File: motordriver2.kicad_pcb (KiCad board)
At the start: 2 copper layers, 99.7 x 79.7 mm, 129 parts, among them J1 Conn_01x02_Pin, J2 SUB-DRAM-602A-002, J3 SUB-DRAM-602A-002, J4 Conn_01x06_Pin, J5 Conn_01x03_Pin, M1 Motor_DC, Q1 TPHR9003NL, Q2 TPHR9003NL, Q3 TPHR9003NL, Q4 TPHR9003NL, SW1 TS-1187A-B-A-B, SW2 TS-1187A-B-A-B, SW3 TS-1187A-B-A-B, SW4 TS-1187A-B-A-B, SW5 TS-1187A-B-A-B, U1 SN65HVD234, U2 PLM2105DR, U3 STM32F302C8Tx, U4 24LC256, U5 PLM2105DR, U6 AMS1117-3.3, U7 AMS1117-3.3, Y1 Q13FC1350000400, Y2 X322516MLB4SI

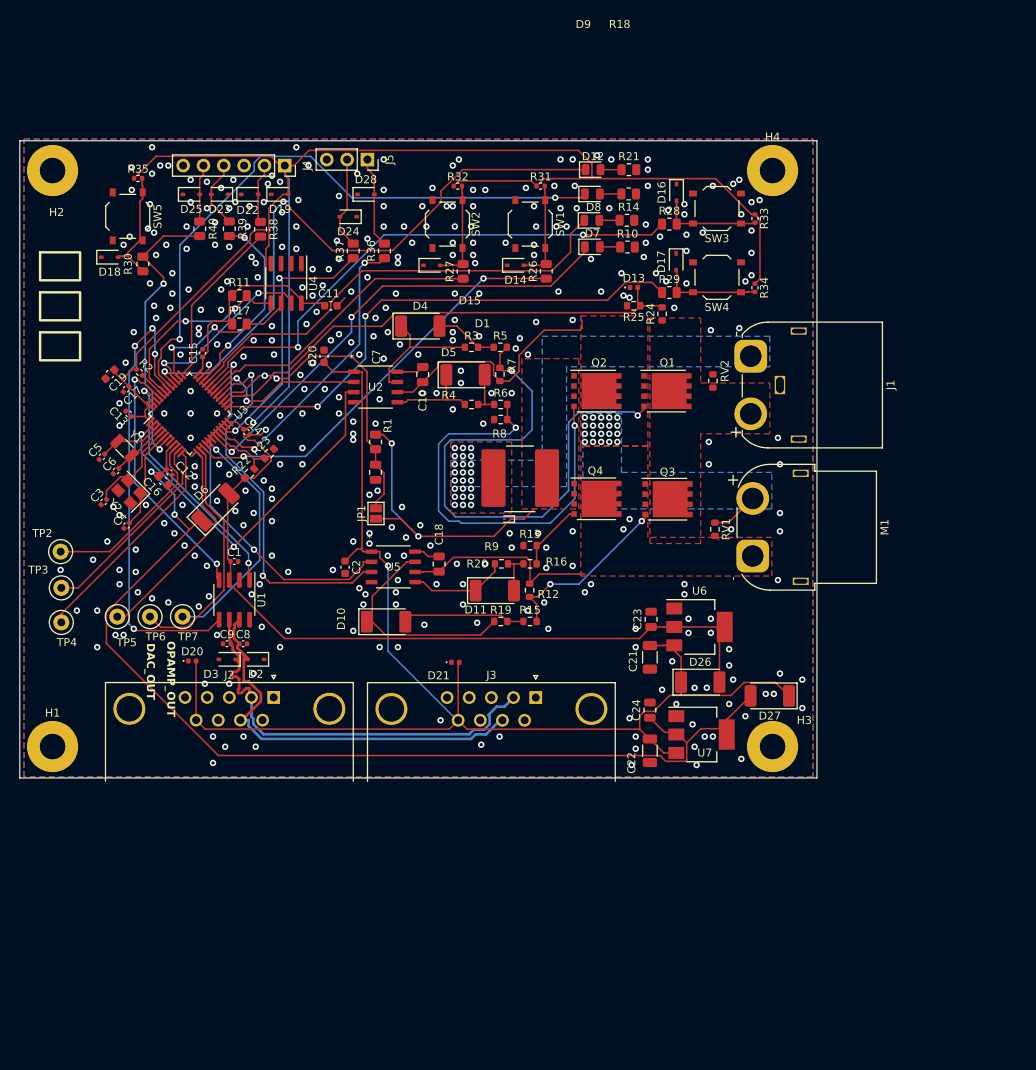
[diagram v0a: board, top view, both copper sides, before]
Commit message: change
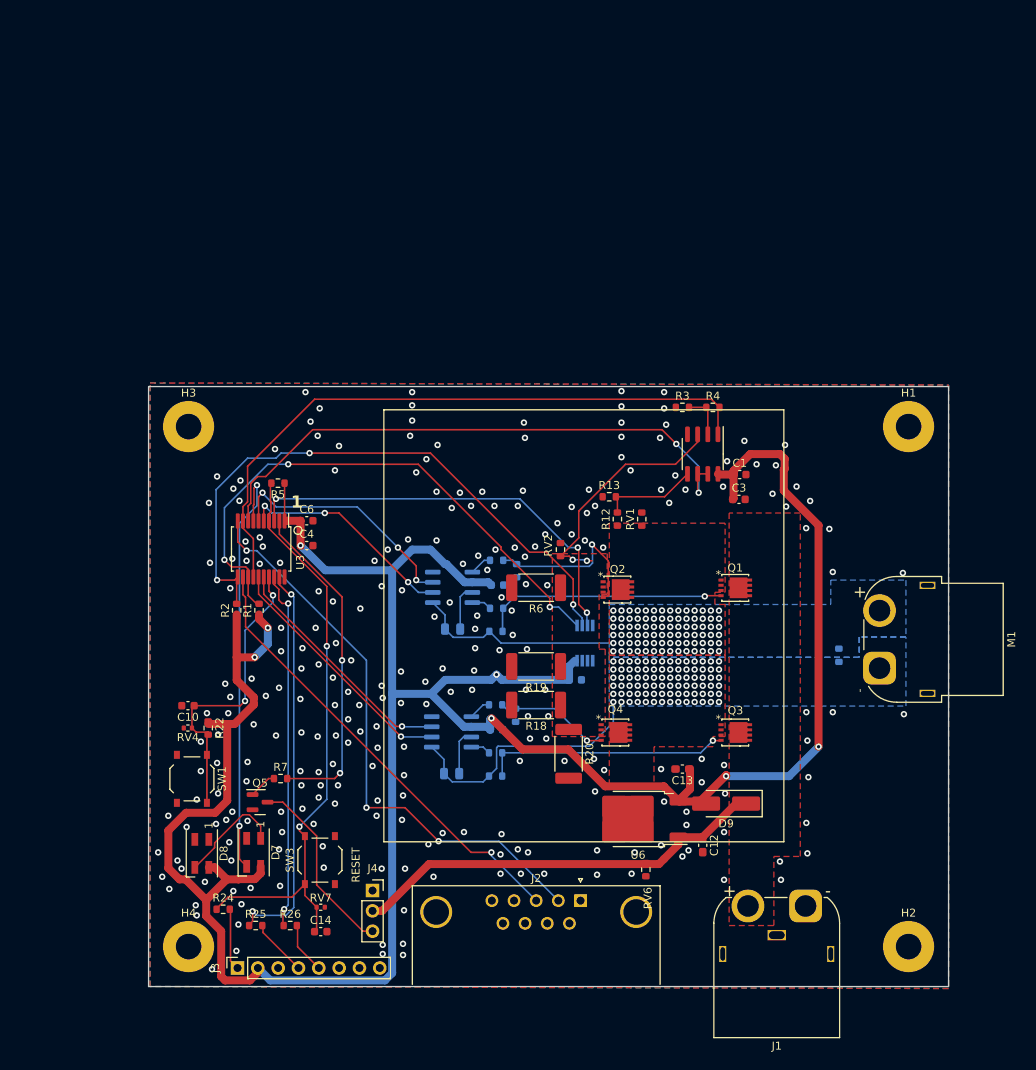
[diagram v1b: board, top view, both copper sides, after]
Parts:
- removed C16, C20: CL10A105KB8NNNC, Capacitor_SMD:C_0603_1608Metric
- removed C17: CL05B104KO5NNNC, Capacitor_SMD:C_0402_1005Metric
- removed C18: CL21B224KBFNNNE, Capacitor_SMD:C_0805_2012Metric
- removed C19: CL10A475KO8NNNC, Capacitor_SMD:C_0603_1608Metric
- removed C21, C22: CL31B105KBHNNNE, Capacitor_SMD:C_1206_3216Metric
- removed C23, C24: CL21A226MAQNNNE, Capacitor_SMD:C_0805_2012Metric
- removed C7: CL21C200JBANNNC, Capacitor_SMD:C_0805_2012Metric
- removed C8: 0402CG150J500NT, Capacitor_SMD:C_0402_1005Metric
- removed D1: ESD9X3.3ST5G, Diode_SMD:D_SOD-923
- removed D10, D11, D26, D27, D4, D5, D6: SS34, Diode_SMD:D_MELF
- removed D12: KT-0805G, Diode_SMD:D_0805_2012Metric
- removed D13, D20, D21: ES0402V014BT, Diode_SMD:D_0402_1005Metric
- removed D14, D15, D16, D17, D18, D19, D2, D22, D23, D24, D25, D28, D3: ESD3Z5.0C, Diode_SMD:D_SOD-323
- removed J5: Conn_01x03_Pin, Connector_PinSocket_2.54mm:PinSocket_1x03_P2.54mm_Vertical
- removed JP1: Jumper_2_Open, Jumper:SolderJumper-2_P1.3mm_Open_Pad1.0x1.5mm
- removed R21: 0805W8F1000T5E, Resistor_SMD:R_0805_2012Metric
- removed R23: 0603WAF7501T5E, Resistor_SMD:R_0603_1608Metric
- removed R27, R28, R29, R30, R36, R37, R38, R39, R40: 0805W8F100JT5E, Resistor_SMD:R_0805_2012Metric
- removed R31, R32, R33, R34, R35: 0402WGF1002TCE, Resistor_SMD:R_0402_1005Metric
- removed SW2, SW4, SW5: TS-1187A-B-A-B, Button_Switch_SMD:SW_Push_1P1T_XKB_TS-1187A
- removed TP2, TP3, TP4, TP5, TP6, TP7: TestPoint, TestPoint:TestPoint_Loop_D1.80mm_Drill1.0mm_Beaded
- removed U4: 24LC256, Package_SO:SOIC-8_3.9x4.9mm_P1.27mm
- removed Y1: Q13FC1350000400, Crystal:Crystal_SMD_3215-2Pin_3.2x1.5mm
- removed Y2: X322516MLB4SI, Crystal:Crystal_SMD_3225-4Pin_3.2x2.5mm
- added Q5: AO3400A, Package_TO_SOT_SMD:SOT-23, F.Cu at (88.9, 166.9)
- added RV3: SDV1608H260C050YPTF, Resistor_SMD:R_0603_1608Metric, B.Cu at (161.3, 148.6)
- added RV4: AVR-M1005C080MTADB, Resistor_SMD:R_0402_1005Metric, F.Cu at (79.9, 157.7)
- added RV6: SDV1608H260C050YPTF, Resistor_SMD:R_0603_1608Metric, F.Cu at (137.2, 175.4)
- added RV7: AVR-M1005C080MTADB, Resistor_SMD:R_0402_1005Metric, F.Cu at (96.5, 180.1)
- C1: value CL05B104KO5NNNC -> CL10A106KP8NNNC; footprint Capacitor_SMD:C_0402_1005Metric -> Capacitor_SMD:C_0603_1608Metric
- C10: value CL21B224KBFNNNE -> CC0603KRX7R9BB104; footprint Capacitor_SMD:C_0805_2012Metric -> Capacitor_SMD:C_0603_1608Metric
- C11: value CL10A475KO8NNNC -> CL10A105KB8NNNC; moved to B.Cu
- C12: value CL05B103KB5NNNC -> CL10A105KB8NNNC; footprint Capacitor_SMD:C_0402_1005Metric -> Capacitor_SMD:C_0603_1608Metric_Pad1.08x0.95mm_HandSolder
- C13: value CL05B104KO5NNNC -> CL21A226MAQNNNE; footprint Capacitor_SMD:C_0402_1005Metric -> Capacitor_SMD:C_0603_1608Metric_Pad1.08x0.95mm_HandSolder
- C14: value CL05B104KO5NNNC -> CC0603KRX7R9BB104; footprint Capacitor_SMD:C_0402_1005Metric -> Capacitor_SMD:C_0603_1608Metric
- C15: value CL05B104KO5NNNC -> CL21B224KBFNNNE; footprint Capacitor_SMD:C_0402_1005Metric -> Capacitor_SMD:C_0805_2012Metric; moved to B.Cu
- C2, R16: moved to B.Cu
- C3: value CL05C100JB5NNNC -> CC0603KRX7R9BB104; footprint Capacitor_SMD:C_0402_1005Metric -> Capacitor_SMD:C_0603_1608Metric
- C4: value CL05C100JB5NNNC -> CL10A106KP8NNNC; footprint Capacitor_SMD:C_0402_1005Metric -> Capacitor_SMD:C_0603_1608Metric
- C5: value 0402CG150J500NT -> CL21B224KBFNNNE; footprint Capacitor_SMD:C_0402_1005Metric -> Capacitor_SMD:C_0805_2012Metric; moved to B.Cu
- C6: value 0402CG150J500NT -> CC0603KRX7R9BB104; footprint Capacitor_SMD:C_0402_1005Metric -> Capacitor_SMD:C_0603_1608Metric
- C9: value 0402CG150J500NT -> CC0603KRX7R9BB104; footprint Capacitor_SMD:C_0402_1005Metric -> Capacitor_SMD:C_0603_1608Metric; moved to B.Cu
- D7, D8: value NCD0805R1 -> SK6812MINI; footprint Diode_SMD:D_0805_2012Metric -> LED_SMD:LED_SK6812MINI_PLCC4_3.5x3.5mm_P1.75mm
- D9: value KT-0805Y -> RS1M; footprint Diode_SMD:D_0805_2012Metric -> Diode_SMD:D_SMA_Handsoldering
- J2: value SUB-DRAM-602A-002 -> DMR-09PGG
- J3: value SUB-DRAM-602A-002 -> ICSP; footprint Connector_Dsub:DSUB-9_Female_Horizontal_P2.77x2.84mm_EdgePinOffset7.70mm_Housed_MountingHolesOffset9.12mm -> Connector_PinSocket_2.54mm:PinSocket_1x08_P2.54mm_Vertical
- J4: value Conn_01x06_Pin -> FAN; footprint Connector_PinSocket_2.54mm:PinSocket_1x06_P2.54mm_Vertical -> Connector_PinSocket_2.54mm:PinSocket_1x03_P2.54mm_Vertical
- Q1, Q2, Q3, Q4: value TPHR9003NL -> TPN1R603PLL1Q; footprint Package_SON:VSONP-8-1EP_5x6_P1.27mm -> 000localproj:TSON Advance_TOS
- R1: value 0805W8F100JT5E -> 0402WGF1002TCE; footprint Resistor_SMD:R_0805_2012Metric -> Resistor_SMD:R_0603_1608Metric
- R10, R14: value 0805W8F1000T5E -> 0603WAF1002T5E; footprint Resistor_SMD:R_0805_2012Metric -> Resistor_SMD:R_0603_1608Metric; moved to B.Cu
- R11: value 0805W8F3301T5E -> 0603WAF1002T5E; footprint Resistor_SMD:R_0805_2012Metric -> Resistor_SMD:R_0603_1608Metric; moved to B.Cu
- R12: value 0603WAF1002T5E -> 0603WAF5102T5E
- R13: value 0603WAF1002T5E -> 0603WAF1801T5E
- R15: value 0603WAF470JT5E -> 0603WAF1002T5E; moved to B.Cu
- R17: value 0805W8F3301T5E -> 0603WAF470JT5E; footprint Resistor_SMD:R_0805_2012Metric -> Resistor_SMD:R_0603_1608Metric; moved to B.Cu
- R18: value 0805W8F1000T5E -> 0.008; footprint Resistor_SMD:R_0805_2012Metric -> Resistor_SMD:R_2512_6332Metric_Pad1.40x3.35mm_HandSolder
- R19, R20, R6: value 0603WAF470JT5E -> 0.008; footprint Resistor_SMD:R_0603_1608Metric -> Resistor_SMD:R_2512_6332Metric_Pad1.40x3.35mm_HandSolder
- R2: footprint Resistor_SMD:R_0402_1005Metric -> Resistor_SMD:R_0603_1608Metric
- R22: value 0603WAF3601T5E -> 0402WGF1002TCE
- R24: value 0603WAF1802T5E -> 0805W8F100JT5E
- R25: value 0603WAF2001T5E -> 0805W8F100JT5E
- R26: footprint Resistor_SMD:R_0805_2012Metric -> Resistor_SMD:R_0603_1608Metric
- R3: value 0603WAF470JT5E -> 0603WAF9101T5E
- R4: value 0603WAF470JT5E -> 0603WAF7502T5E
- R5: value 0603WAF470JT5E -> 0402WGF1002TCE
- R7: value 0603WAF1002T5E -> 0603WAF470JT5E
- R8: value 0603WAF1002T5E -> 0603WAF470JT5E; moved to B.Cu
- R9: value HoXLR2728D-4W-7mR-1% -> 0603WAF470JT5E; footprint 000localproj:R_2728_7142Metric -> Resistor_SMD:R_0603_1608Metric; moved to B.Cu
- U1: value SN65HVD234 -> LM358
- U2: value PLM2105DR -> MCP14700T-E/SN; footprint 000localproj:SOIC8_D_TEX -> Package_SO:SOIC-8_3.9x4.9mm_P1.27mm; moved to B.Cu
- U3: value STM32F302C8Tx -> PIC16F1829-ISS; footprint Package_QFP:LQFP-48_7x7mm_P0.5mm -> Package_SO:SSOP-20_5.3x7.2mm_P0.65mm
- U5: value PLM2105DR -> TMP1075DGK; footprint 000localproj:SOIC8_D_TEX -> Package_SO:VSSOP-8_3.0x3.0mm_P0.65mm; moved to B.Cu
- U6: value AMS1117-3.3 -> L78M05ABDT-TR; footprint Package_TO_SOT_SMD:SOT-223-3_TabPin2 -> Package_TO_SOT_SMD:TO-252-2
- U7: value AMS1117-3.3 -> MCP14700T-E/SN; footprint Package_TO_SOT_SMD:SOT-223-3_TabPin2 -> Package_SO:SOIC-8_3.9x4.9mm_P1.27mm; moved to B.Cu
- moved H2 144.4 mm to (170.0, 185.0)
- moved H4 121.4 mm to (80.0, 185.0)
- moved H1 114.2 mm to (170.0, 120.0)
- moved SW3 95.4 mm to (96.4, 174.2), turned to 90 degrees
- moved D8 92.9 mm to (81.7, 173.4), turned to -90 degrees
- moved R24 92.5 mm to (84.3, 180.3), turned to 0 degrees
- moved J4 91.3 mm to (103.0, 178.0), turned to 0 degrees
- moved R25 90.7 mm to (88.4, 182.4), turned to 0 degrees
- moved R26 87.8 mm to (92.7, 182.4), turned to 0 degrees
- moved D7 86.7 mm to (88.1, 173.2), turned to -90 degrees
- moved H3 83.2 mm to (80.0, 120.0)
- moved C13 82.2 mm to (141.7, 162.8), turned to 180 degrees
- moved C12 81.4 mm to (144.3, 172.3), turned to -90 degrees
- moved SW1 81.2 mm to (80.4, 164.0)
- moved C3 79.4 mm to (148.8, 129.1), turned to 0 degrees
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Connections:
- C1 pad 1: +3.3V -> +5V
- C10 pad 1: Net-(M1--) -> /IN1
- C10 pad 2: Net-(U2-BST) -> GND
- C11 pad 1: +3.3V -> +5V
- C12 pad 1: +3.3VA -> VDD
- C13 pad 1: +3.3V -> +5V
- C14 pad 1: +3.3V -> /MCLR*
- C15 pad 1: +3.3V -> Net-(M1-+)
- C15 pad 2: GND -> Net-(U7-BOOT)
- C2 pad 1: +12V -> +5V
- C3 pad 1: GND -> +5V
- C3 pad 2: Net-(U3-PF0) -> GND
- C4 pad 1: GND -> +5V
- C4 pad 2: Net-(U3-PF1) -> GND
- C5 pad 1: GND -> /voltage_motor
- C5 pad 2: Net-(U3-PC14) -> Net-(U2-BOOT)
- C6 pad 1: GND -> +5V
- C6 pad 2: Net-(U3-PC15) -> GND
- C9 pad 1: GND -> +5V
- C9 pad 2: /CAN_N -> GND
- D7 pad 1: /COMP4_OUT -> Net-(D7-DOUT)
- D7 pad 2: Net-(D7-A) -> GND
- D8 pad 1: /COMP2_OUT -> unconnected-(D8-DOUT-Pad1)
- D8 pad 2: Net-(D8-A) -> GND
- D9 pad 1: /IO_OUT4 -> VDD
- D9 pad 2: Net-(D9-A) -> +5V
- J2 pad 2: /CAN_N -> /PIC_UART_TX
- J2 pad 3: GND -> /PIC_UART_RX
- J2 pad 7: /CAN_P -> unconnected-(J2-Pad7)
- J2 pad 9: +12V -> unconnected-(J2-Pad9)
- J3 pad 1: unconnected-(J3-Pad1) -> Net-(J3-Pin_1)
- J3 pad 2: /CAN_N -> +5V
- J3 pad 4: unconnected-(J3-Pad4) -> Net-(J3-Pin_4)
- J3 pad 5: GND -> Net-(J3-Pin_5)
- J3 pad 6: GND -> unconnected-(J3-Pin_6-Pad6)
- J3 pad 7: /CAN_P -> unconnected-(J3-Pin_7-Pad7)
- J4 pad 1: +3.3V -> unconnected-(J4-Pin_1-Pad1)
- J4 pad 2: Net-(D22-A2) -> VDD
- J4 pad 3: GND -> Net-(J4-Pin_3)
- M1 pad 2: Net-(M1--) -> /voltage_motor
- Q1 pad 1: Net-(M1--) -> /voltage_motor
- Q2 pad 3: Net-(M1--) -> /voltage_motor
- R1 pad 1: /VSen -> +5V
- R1 pad 2: Net-(JP1-B) -> /SDA
- R10 pad 1: Net-(D7-A) -> /voltage_motor
- R10 pad 2: GND -> Net-(Q1-G)
- R11 pad 1: +3.3V -> GND
- R11 pad 2: /I2C_SDA -> Net-(Q2-G)
- R12 pad 1: Net-(M1-+) -> /voltage_motor
- R12 pad 2: Net-(Q3-G) -> Net-(U1B-+)
- R13 pad 2: Net-(Q4-G) -> Net-(U1B-+)
- R14 pad 1: Net-(D8-A) -> Net-(M1-+)
- R14 pad 2: GND -> Net-(Q3-G)
- R15 pad 1: Net-(D10-A) -> GND
- R15 pad 2: Net-(Q3-G) -> Net-(Q4-G)
- R16 pad 1: Net-(D11-A) -> Net-(U7-HIGHDR)
- R16 pad 2: Net-(Q4-G) -> Net-(Q3-G)
- R17 pad 1: +3.3V -> Net-(U7-LOWDR)
- R17 pad 2: /I2C_SCL -> Net-(Q4-G)
- R18 pad 1: Net-(D9-A) -> /VSen
- R19 pad 1: Net-(D10-K) -> /VSen
- R19 pad 2: Net-(D10-A) -> GND
- R2 pad 1: +3.3V -> +5V
- R2 pad 2: Net-(U3-BOOT0) -> /SCL
- R20 pad 1: Net-(D11-K) -> /VSen
- R20 pad 2: Net-(D11-A) -> GND
- R22 pad 1: +3.3V -> +5V
- R22 pad 2: /COMP4_INM -> /IN1
- R24 pad 1: VDD -> /MCLR*
- R24 pad 2: /ADC1_IN13 -> Net-(J3-Pin_1)
- R25 pad 1: /ADC1_IN13 -> /PGD
- R25 pad 2: GND -> Net-(J3-Pin_4)
- R26 pad 1: /IO_IN1 -> /PGC
- R26 pad 2: Net-(D14-A2) -> Net-(J3-Pin_5)
- R3 pad 1: Net-(D4-K) -> GND
- R3 pad 2: Net-(D4-A) -> /IN2
- R4 pad 1: Net-(D5-K) -> /IN2
- R4 pad 2: Net-(D5-A) -> /ISenseIN
- R5 pad 1: Net-(D4-A) -> +5V
- R5 pad 2: Net-(Q1-G) -> /MCLR*
- R6 pad 1: Net-(D5-A) -> /VSen
- R6 pad 2: Net-(Q2-G) -> GND
- R7 pad 1: Net-(M1--) -> Net-(Q5-G)
- R7 pad 2: Net-(Q1-G) -> /FAN
- R8 pad 1: GND -> Net-(U2-HIGHDR)
- R8 pad 2: Net-(Q2-G) -> Net-(Q1-G)
- R9 pad 1: /VSen -> Net-(U2-LOWDR)
- R9 pad 2: GND -> Net-(Q2-G)
- RV1 pad 1: Net-(M1--) -> /voltage_motor
- RV1 pad 2: Net-(M1-+) -> GND
- RV2 pad 1: VDD -> GND
- RV2 pad 2: GND -> /VSen
- SW1 pad 1: Net-(D14-A2) -> /IN1
- SW3 pad 1: Net-(D16-A2) -> /MCLR*
- U1 pad 1: /CAN_TX_STM -> /ISenseIN
- U1 pad 2: GND -> /IN2
- U1 pad 3: +3.3V -> /VSen
- U1 pad 4: /CAN_RX_STM -> GND
- U1 pad 5: /IO_OUT2 -> Net-(U1B-+)
- U1 pad 6: /CAN_N -> /VSenseIN
- U1 pad 7: /CAN_P -> /VSenseIN
- U1 pad 8: GND -> +5V
- U2 pad 1: +12V -> /voltage_motor
- U2 pad 5: Net-(D5-K) -> Net-(U2-LOWDR)
- U2 pad 6: Net-(M1--) -> +5V
- U2 pad 7: Net-(D4-K) -> Net-(U2-BOOT)
- U2 pad 8: Net-(U2-BST) -> Net-(U2-HIGHDR)
- U3 pad 1: +3.3V -> +5V
- U3 pad 10: Net-(U3-PA0) -> /PIC_UART_TX
- U3 pad 11: Net-(U3-PA1) -> /SCL
- U3 pad 12: Net-(U3-PA2) -> /PIC_UART_RX
- U3 pad 13: Net-(U3-PA3) -> /SDA
- U3 pad 14: /DAC_OUT -> /ISenseIN
- U3 pad 15: /IO_IN1 -> /GATEHB
- U3 pad 16: /OPAMP_OUT -> /GATELB
- U3 pad 17: /OPAMP_OUT -> /IN1
- U3 pad 18: /OPAMP_OUT -> /PGC
- U3 pad 19: /COMP4_OUT -> /PGD
- U3 pad 2: /GATELA -> /FAN
- U3 pad 20: /COMP4_INM -> GND
- U3 pad 3: Net-(U3-PC14) -> /INT
- U3 pad 4: Net-(U3-PC15) -> /MCLR*
- U3 pad 5: Net-(U3-PF0) -> /GATEHA
- U3 pad 6: Net-(U3-PF1) -> /GATELA
- U3 pad 7: /NRST -> /LED
- U3 pad 8: GND -> /VSenseIN
- U3 pad 9: +3.3VA -> /ISenseIN
- U5 pad 1: +12V -> /SDA
- U5 pad 2: /GATEHB -> /SCL
- U5 pad 3: /GATELB -> /INT
- U5 pad 5: Net-(D11-K) -> GND
- U5 pad 6: Net-(M1-+) -> GND
- U5 pad 7: Net-(D10-K) -> GND
- U5 pad 8: Net-(U5-BST) -> +5V
- U6 pad 1: GND -> VDD
- U6 pad 2: +3.3V -> GND
- U6 pad 3: +12V -> +5V
- U7 pad 1: GND -> Net-(M1-+)
- U7 pad 2: +3.3VA -> /GATEHB
- U7 pad 3: +12V -> /GATELB
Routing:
- net +5V: track 0.00 -> 331.7 mm, vias 0 -> 7
- net +3.3V: track 330.3 -> 0.00 mm, vias 1 -> 0
- net +12V: track 167.8 -> 0.00 mm, vias 1 -> 0
- net +3.3VA: track 135.0 -> 0.00 mm, vias 2 -> 0
- net /ISenseIN: track 0.00 -> 80.9 mm
- net /IO_OUT3: track 78.4 -> 0.00 mm, vias 2 -> 0
- net /IO_OUT4: track 78.1 -> 0.00 mm, vias 2 -> 0
- net /SCL: track 0.00 -> 77.2 mm, vias 0 -> 3
- net /MCLR*: track 0.00 -> 74.2 mm, vias 0 -> 2
- net /VSenseIN: track 0.00 -> 72.5 mm, vias 0 -> 2
- net /PIC_UART_TX: track 0.00 -> 72.0 mm, vias 0 -> 3
- net /SDA: track 0.00 -> 70.7 mm, vias 0 -> 3
- net /TIM1_BKIN2: track 67.3 -> 0.00 mm, vias 2 -> 0
- net /TIM1_BKIN: track 64.3 -> 0.00 mm, vias 2 -> 0
- net /ADC1_IN13: track 62.2 -> 0.00 mm
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- added copper zone on B.Cu, net /voltage_motor
- added copper zone on F.Cu, net /voltage_motor
- added copper zone on B.Cu, net Net-(M1-+)
- removed copper zone on B.Cu, net Net-(M1--)
- removed copper zone on F.Cu, net Net-(M1--)
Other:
- board size 99.7 x 79.7 mm -> 100 x 75 mm
- board text added: "1"
- board text added: "2024-misohiyoko-Gentaro KODAMA"
- board text added: "JLCPCB"
- board text added: "RESET"
- board text removed: "DAC_OUT"
- board text removed: "OPAMP_OUT"
- board text removed: "Q3"
